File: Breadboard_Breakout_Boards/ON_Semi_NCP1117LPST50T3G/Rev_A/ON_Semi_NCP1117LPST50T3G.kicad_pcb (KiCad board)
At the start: 2 copper layers, 11.2 x 7.4 mm, 2 parts, among them J1 PinHeader_1x03_P2.54mm_Vertic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, U1 ON_Semi_NCP1117LPST50T3G

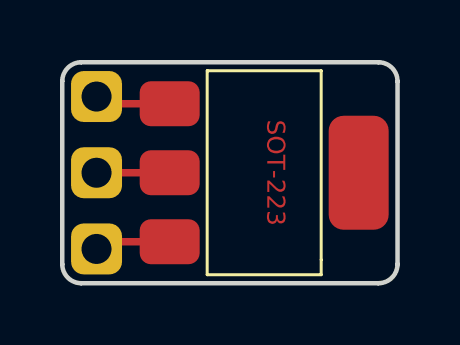
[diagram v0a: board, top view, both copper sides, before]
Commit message: Revision A boards checked before sending off to fab
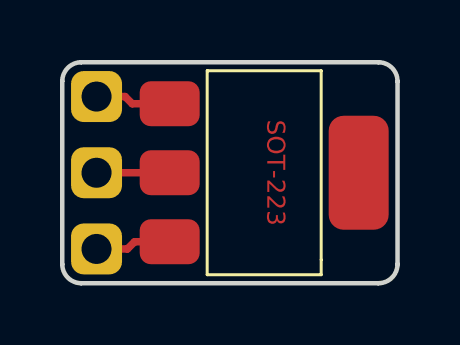
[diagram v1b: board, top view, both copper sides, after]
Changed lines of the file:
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@@
     (thickness 1.6)
     (drawings 13)
-    (tracks 5)
+    (tracks 8)
     (zones 0)
     (modules 2)
@@
     (pad_drill 0.762)
     (pad_to_mask_clearance 0.0508)
-    (solder_mask_min_width 0.0508)
     (aux_axis_origin 0 0)
     (visible_elements 7FFFFFFF)
@@
   )
   (segment (start 157.085 88.505) (end 156.845 88.265) (width 0.25) (layer F.Cu) (net 1))
-  (segment (start 159.283 88.505) (end 157.085 88.505) (width 0.25) (layer F.Cu) (net 1))
-  (segment (start 157.085 93.105) (end 156.845 93.345) (width 0.25) (layer F.Cu) (net 2))
-  (segment (start 159.283 93.105) (end 157.085 93.105) (width 0.25) (layer F.Cu) (net 2))
+  (segment (start 157.795 88.265) (end 156.845 88.265) (width 0.25) (layer F.Cu) (net 1))
+  (segment (start 159.283 88.505) (end 158.035 88.505) (width 0.25) (layer F.Cu) (net 1))
+  (segment (start 158.035 88.505) (end 157.795 88.265) (width 0.25) (layer F.Cu) (net 1))
+  (segment (start 157.875 93.345) (end 156.845 93.345) (width 0.25) (layer F.Cu) (net 2))
+  (segment (start 159.283 93.105) (end 158.115 93.105) (width 0.25) (layer F.Cu) (net 2))
+  (segment (start 158.115 93.105) (end 157.875 93.345) (width 0.25) (layer F.Cu) (net 2))
   (segment (start 159.283 90.805) (end 156.845 90.805) (width 0.25) (layer F.Cu) (net 3))
 )
